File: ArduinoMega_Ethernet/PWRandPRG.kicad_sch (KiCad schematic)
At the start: 98 parts, among them J1 RJ45_Amphenol_RJMG1BD3B8K1ANR, J11 Micro_SD_Card_Det_Hirose_DM3AT, J7 EXT_3V3_I2C, J9 PROGRAM_POWER_USBC, U10 TXS0108EPW, U2 CH340C, U3 ISM330DHCX, U4 W5500, U5 AP63205WU, U6 AP63203WU, U7 SE050C2HQ1, U8 AP22804AW5, U9 MCP7940N-xST, Y2 25Mhz, Y3 32.768kHz

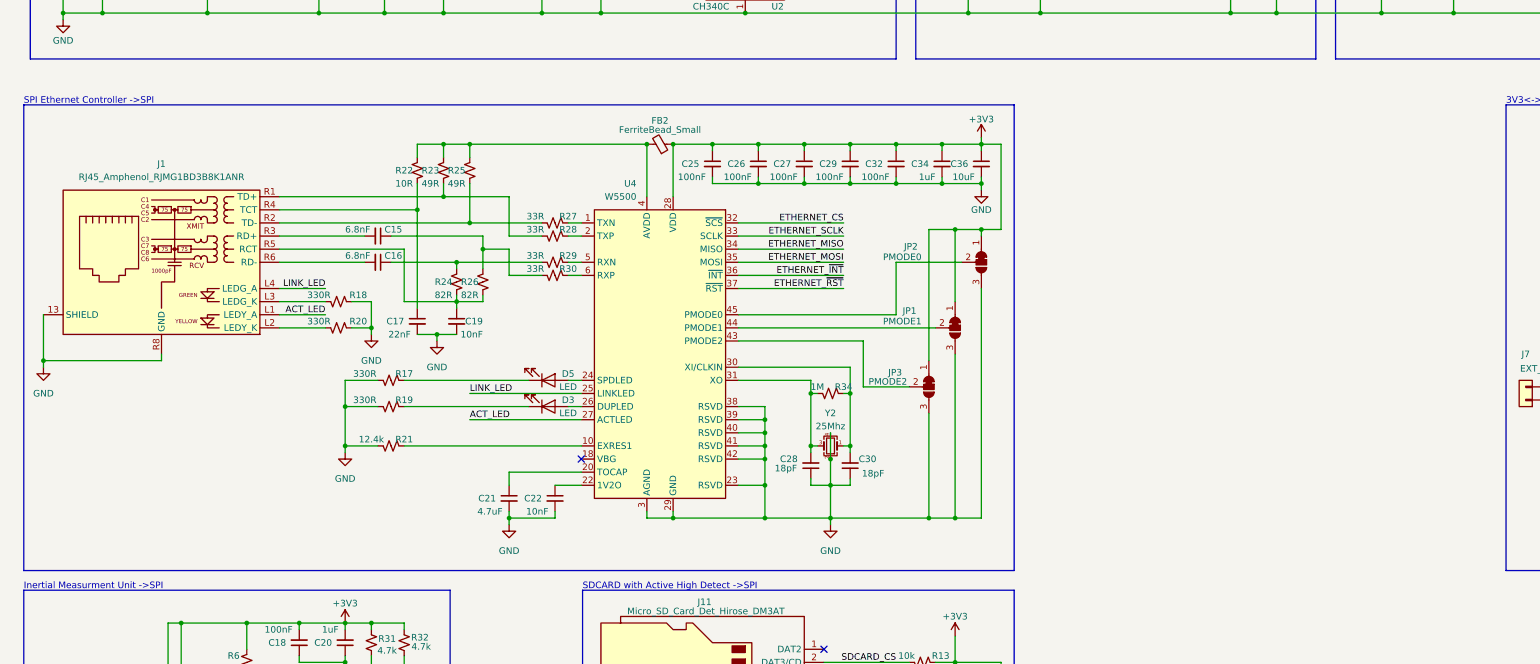
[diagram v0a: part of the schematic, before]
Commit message: w6100 manufacturing and project files
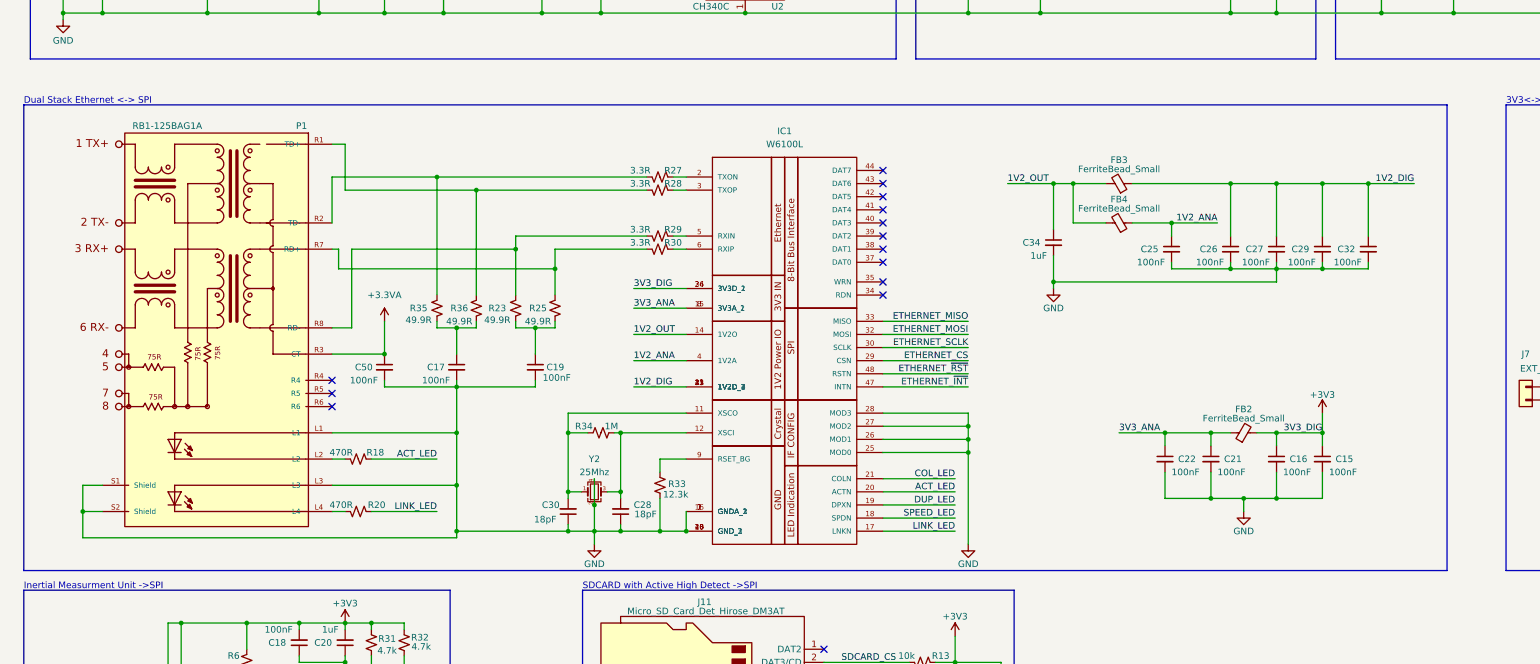
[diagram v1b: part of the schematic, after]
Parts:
- removed C36: 10uF, Capacitor_SMD:C_0805_2012Metric_Pad1.18x1.45mm_HandSolder, symbol Device:C_Small
- removed D3, D5: LED, LED_SMD:LED_0603_1608Metric, symbol Device:LED
- removed J1: RJ45_Amphenol_RJMG1BD3B8K1ANR, Connector_RJ:RJ45_Amphenol_RJMG1BD3B8K1ANR, symbol Connector:RJ45_Amphenol_RJMG1BD3B8K1ANR
- removed JP1: PMODE1, Jumper:SolderJumper-3_P1.3mm_Bridged12_Pad1.0x1.5mm, symbol Jumper:SolderJumper_3_Bridged12
- removed JP2: PMODE0, Jumper:SolderJumper-3_P1.3mm_Bridged12_Pad1.0x1.5mm, symbol Jumper:SolderJumper_3_Bridged12
- removed JP3: PMODE2, Jumper:SolderJumper-3_P1.3mm_Bridged12_Pad1.0x1.5mm, symbol Jumper:SolderJumper_3_Bridged12
- removed R17, R19: 330R, Resistor_SMD:R_0603_1608Metric, symbol Device:R_Small_US
- removed R21: 12.4k, Resistor_SMD:R_0603_1608Metric, symbol Device:R_Small_US
- removed R22: 10R, Resistor_SMD:R_0603_1608Metric, symbol Device:R_Small_US
- removed R24, R26: 82R, Resistor_SMD:R_0603_1608Metric, symbol Device:R_Small_US
- removed U4: W5500, Package_QFP:LQFP-48_7x7mm_P0.5mm, symbol Interface_Ethernet:W5500
- added C50: 100nF, Capacitor_SMD:C_0603_1608Metric, symbol Device:C_Small
- added FB3, FB4: FerriteBead_Small, Inductor_SMD:L_0603_1608Metric, symbol Device:FerriteBead_Small
- added IC1: W6100L, EXT_ETHERNET:QFP50P900X900X160-48N, symbol EXT_ETHERNET:W6100L
- added P1: RB1-125BAG1A, EXT_ETHERNET:WIZNET_RB1-125BAG1A, symbol EXT_ETHERNET:RB1-125BAG1A
- added R33: 12.3k, Resistor_SMD:R_0603_1608Metric, symbol Device:R_Small_US
- added R35, R36: 49.9R, Resistor_SMD:R_0603_1608Metric, symbol Device:R_Small_US
- C15, C16: value 6.8nF -> 100nF
- C17: value 22nF -> 100nF
- C19, C22: value 10nF -> 100nF
- C21: value 4.7uF -> 100nF; footprint Capacitor_SMD:C_0805_2012Metric_Pad1.18x1.45mm_HandSolder -> Capacitor_SMD:C_0603_1608Metric
- R18, R20: value 330R -> 470R
- R23, R25: value 49R -> 49.9R
- R27, R28, R29, R30: value 33R -> 3.3R
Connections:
- net +3V3: now also C15.1, C16.1, FB2.2, IC1.24 (3V3D_1), IC1.36 (3V3D_2); no longer C25.1, C26.1, C27.1, C29.1, C32.1, C34.1, FB2.1
- net ACT_LED: now also R18.1, IC1.20 (ACTN)
- net ETHERNET_CS: now also IC1.29 (CSN)
- net ETHERNET_MISO: now also IC1.33 (MISO)
- net ETHERNET_MOSI: now also IC1.32 (MOSI)
- net ETHERNET_SCLK: now also IC1.30 (SCLK)
- net ETHERNET_~{INT}: now also IC1.47 (INTN)
- net ETHERNET_~{RST}: now also IC1.48 (RSTN)
- net GND: now also C15.2, C16.2, C50.2, IC1.1 (GNDA_1), IC1.10 (GND_1), IC1.16 (GNDA_3), IC1.23 (GND_2), IC1.25 (MOD0), IC1.26 (MOD1), IC1.27 (MOD2), IC1.28 (MOD3), IC1.46 (GND_3), IC1.7 (GNDA_2), P1.L1, P1.L3, P1.S1 (Shield), P1.S2 (Shield), R33.2; no longer R18.1, R20.1
- net LINK_LED: now also R20.1, IC1.17 (LNKN)
- net at R30.2: now also R25.1, P1.R7 (RD+); no longer C15.1
- net at C30.2, R34.1, Y2.1: now also IC1.11 (XSCO)
- net at R20.2: now also P1.L4
- net at C19.1: now also R23.2, R25.2
- net at C28.2, R34.2, Y2.3: now also IC1.12 (XSCI)
- net 3V3_ANA: now reaches C22.1
- net 3V3_ANA: now also C21.1, FB2.1, IC1.15 (3V3A_2), IC1.8 (3V3A_1)
- net at R18.2: now also P1.L2
- net at R28.2: now also P1.R1 (TD+), R36.1; no longer R23.2
- net at R27.2: now also P1.R2 (TD-), R35.1; no longer R25.2
- net at C17.1: now also R35.2, R36.2
- net at R28.1: now also IC1.3 (TXOP)
- net at R29.2: now also R23.1, P1.R8 (RD-); no longer C16.1
- net at R27.1: now also IC1.2 (TXON)
- net at R29.1: now also IC1.5 (RXIN)
- net at R30.1: now also IC1.6 (RXIP)
- new net: IC1.9 (RSET_BG), R33.1
- new net +3.3VA: C50.1, P1.R3 (CT)
- new net 1V2_ANA: C25.1, FB4.1, IC1.4 (1V2A)
- new net 1V2_DIG: C26.1, C27.1, C29.1, C32.1, FB3.1, IC1.13 (1V2D_1), IC1.22 (1V2D_2), IC1.31 (1V2D_3), IC1.45 (1V2D_4)
- new net 1V2_OUT: C34.1, FB3.2, FB4.2, IC1.14 (1V2O)
- new net COL_LED: IC1.21 (COLN)
- new net DUP_LED: IC1.19 (DPXN)
- new net SPEED_LED: IC1.18 (SPDN)
- no-connect marks 13 -> 25
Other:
- note added: "Dual Stack Ethernet <-> SPI"
- note removed: "SPI Ethernet Controller ->SPI"
- moved on the sheet: C17, C19, C25, C26, C27, C28, C29, C30, C32, C34, FB2, R18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
